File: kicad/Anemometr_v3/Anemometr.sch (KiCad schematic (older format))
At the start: 170 parts, among them J1 TxD, J10 +Z1, J11 +Z2, J12 +Z3, J13 +Z4, J14 -Z1, J15 -Z2, J16 -Z3, J17 -Z4, J18 1 TxD+, J19 2 TxD-, J2 RxD, J20 3 RxD+, J21 4-5, J22 6 RxD-, J23 7-8, J24 Conn_01x01_Female, J25 Conn_01x01_Female, J26 Conn_01x01_Female, J3 SCL, J4 SDA, J5 RST, J6 +EXT, J7 -EXT, J8 SWD, J9 SWC, Q1 5N10, U1 STM32F103C8Tx, U2 TS5A3166DBVR, U3 TS5A3166DBVR, U4 LMR14206, U5 TS5A3166DBVR, U6 NCP1117-3.3, U7 TS5A3166DBVR, U8 MCP1703-3.3, U9 MCP1703-3.3, Y1 CSTCE8M00G52A-R0, Y2 ECS-250-20-33

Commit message: изменено:      kicad/Anemometr_v3/Anemometr-cache.lib 	изменено:      kicad/Anemometr_v3/Anemometr-rescue.lib 	изменено:      kicad/Anemometr_v3/Anemometr.sch 	изменено:      kicad/Anemometr_v3/Anemometr.sch-bak 	изменено:      stm32cubeide/Anemometer/.settings/language.settings.xml
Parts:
- D20, D21: symbol My_Library:TLV3501-2 -> Anemometr-rescue:TLV3501-2-My_Library
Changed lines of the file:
@@
 Connection ~ 5900 3950
 $Comp
-L My_Library:TLV3501-2 D20
+L Anemometr-rescue:TLV3501-2-My_Library D20
 U 1 1 637C998F
 P 10050 1350
@@
 	10150 1600 10200 1600
 $Comp
-L My_Library:TLV3501-2 D21
+L Anemometr-rescue:TLV3501-2-My_Library D21
 U 1 1 638DF360
 P 10050 3150

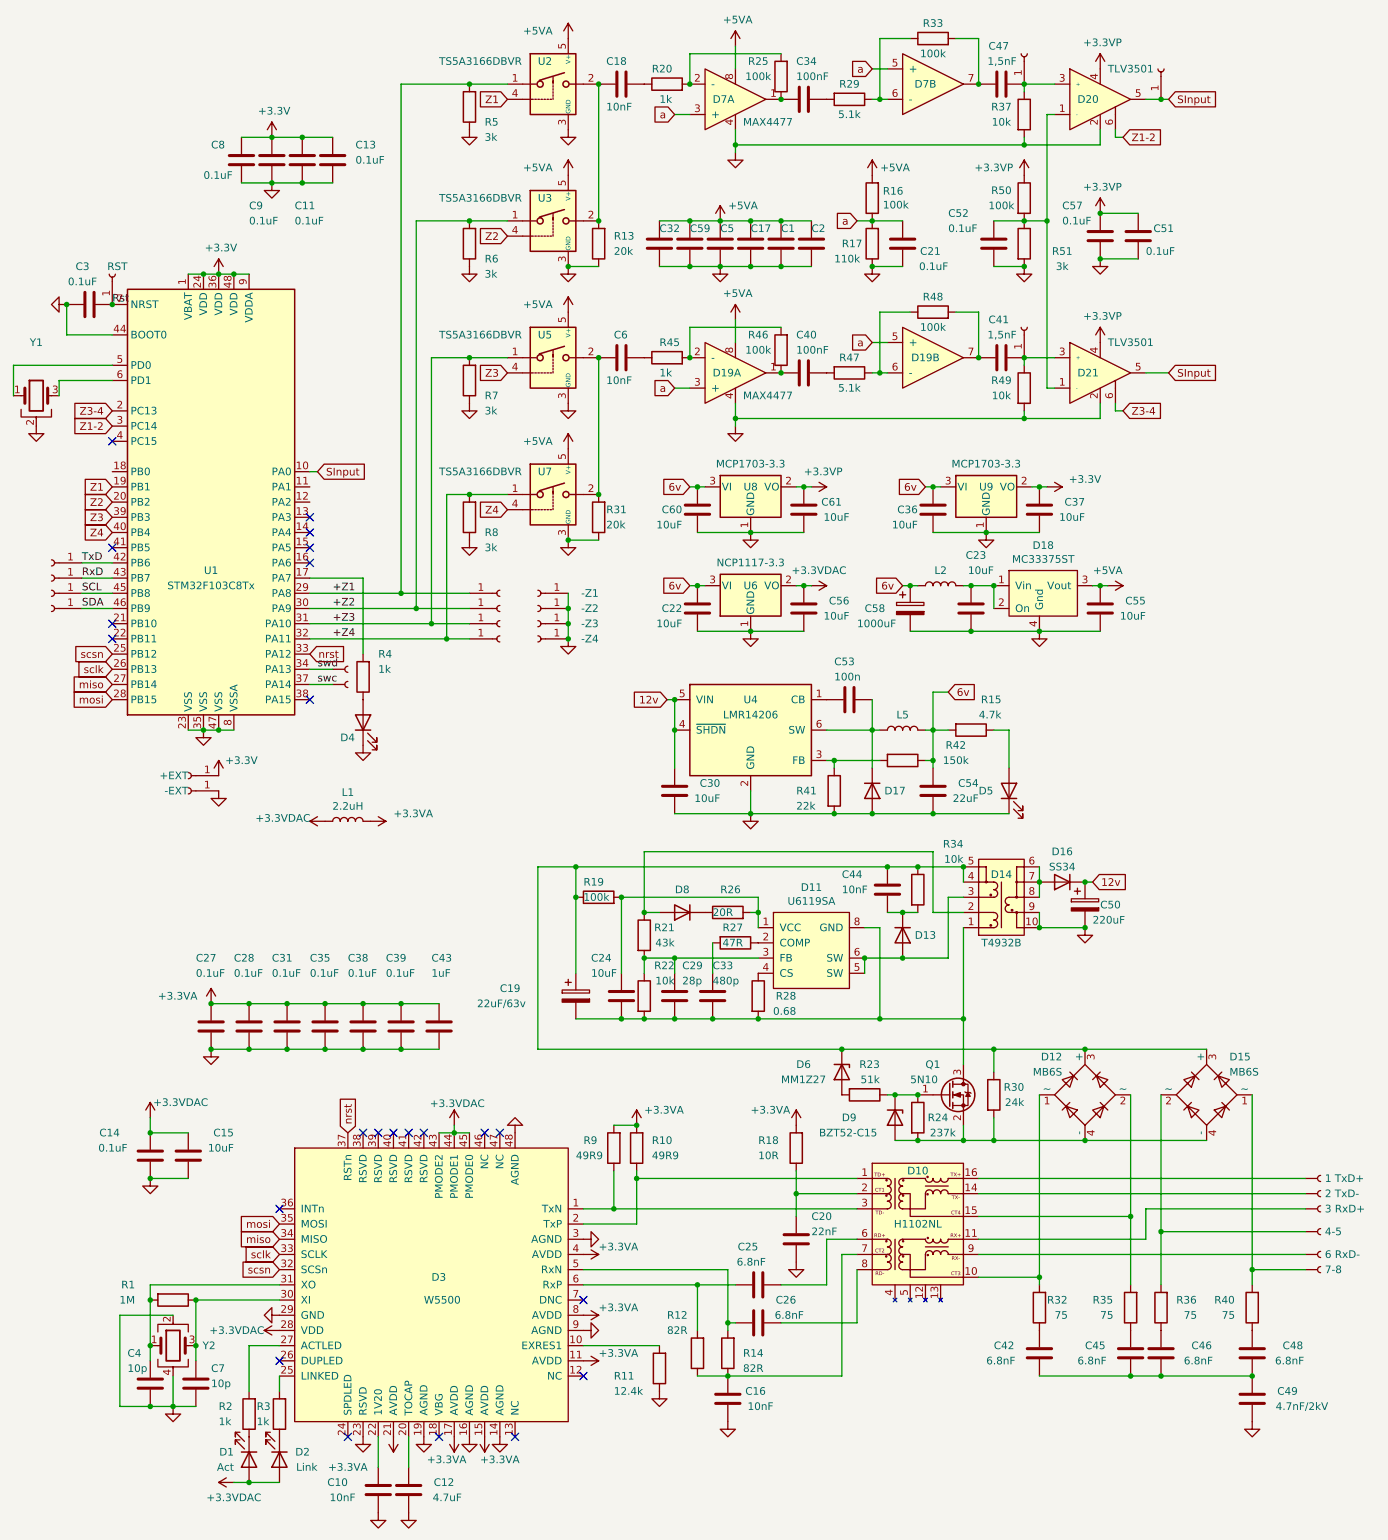
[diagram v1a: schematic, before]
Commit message: изменено:      kicad/Anemometr_v3/Anemometr-cache.lib 	изменено:      kicad/Anemometr_v3/Anemometr.kicad_pcb 	изменено:      kicad/Anemometr_v3/Anemometr.kicad_pcb-bak 	изменено:      kicad/Anemometr_v3/Anemometr.sch 	изменено:      kicad/Anemometr_v3/Anemometr.sch-bak
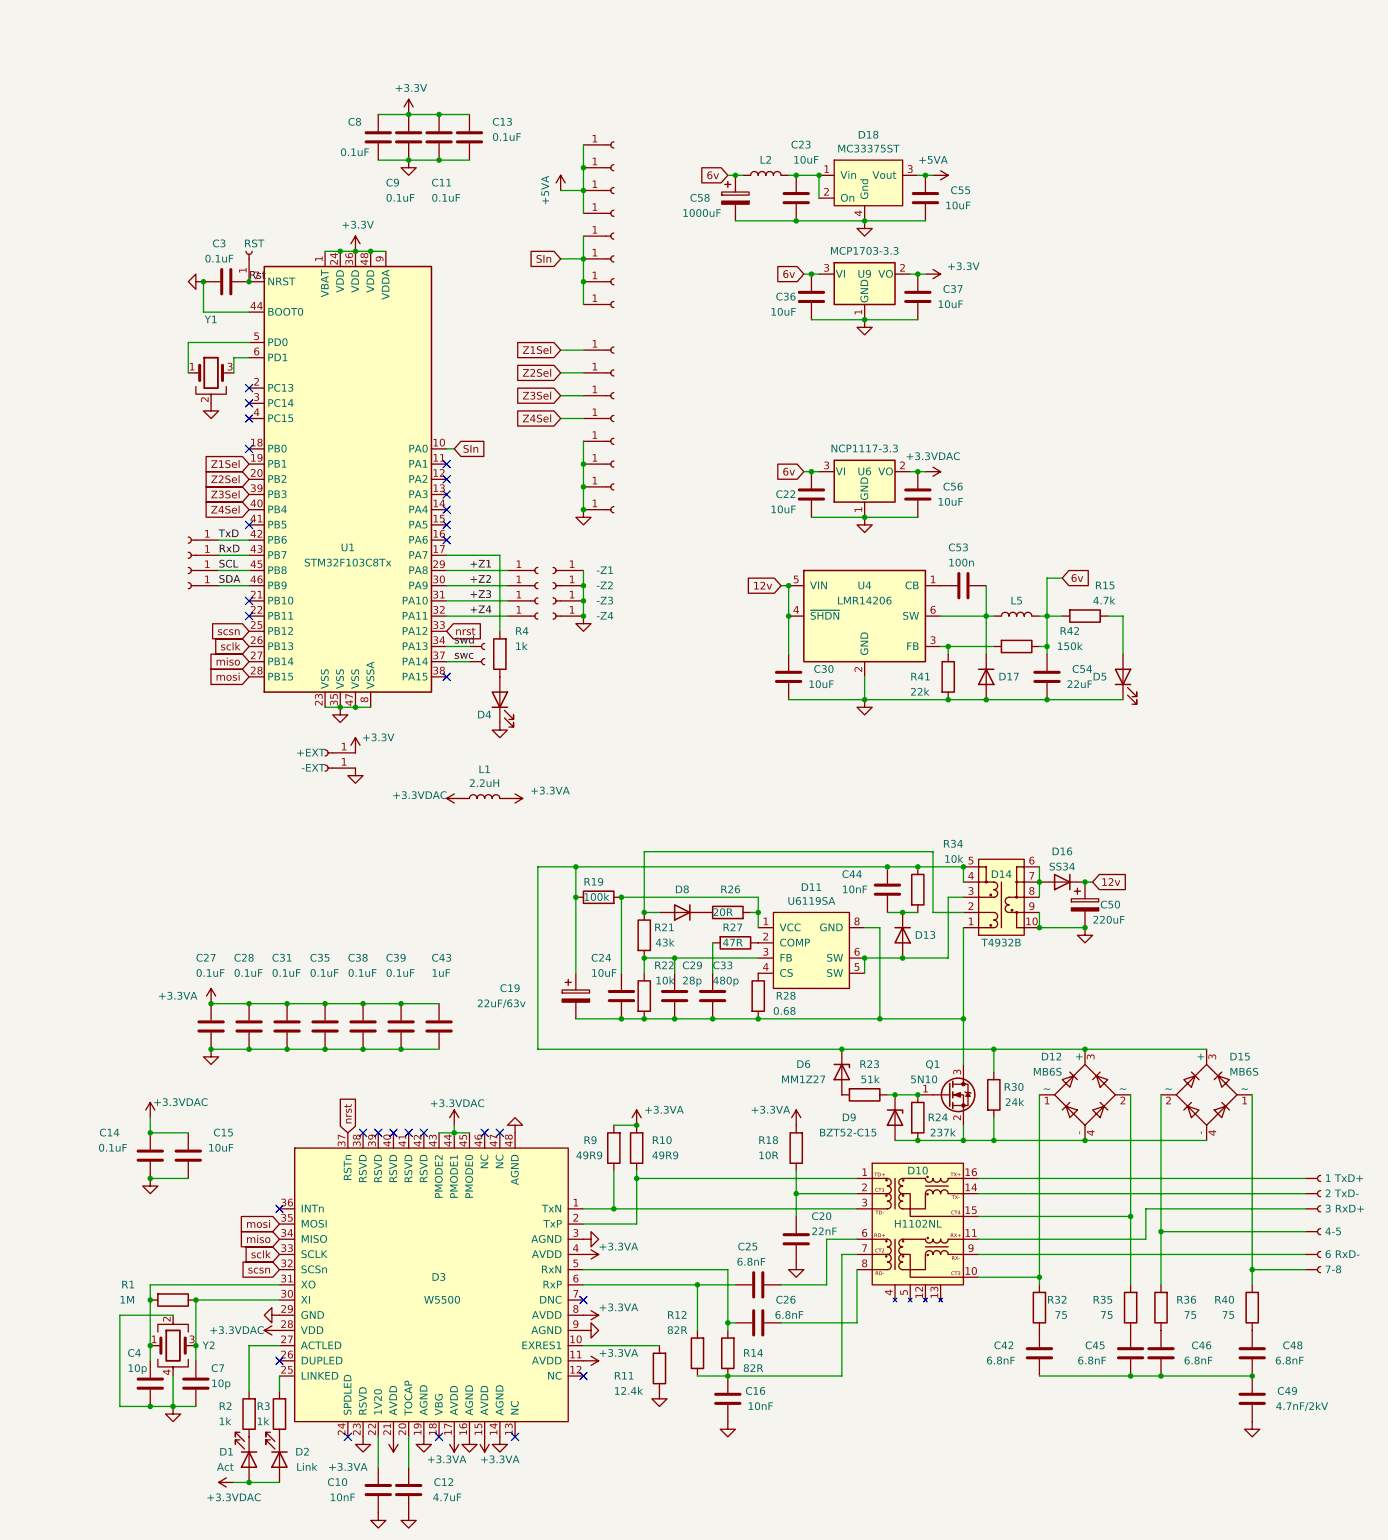
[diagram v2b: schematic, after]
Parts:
- removed C1, C17, C2, C21, C32, C5, C51, C52, C57, C59: 0.1uF, Capacitor_SMD:C_0402_1005Metric, symbol Device:C
- removed C18, C6: 10nF, Capacitor_SMD:C_0402_1005Metric, symbol Device:C
- removed C34, C40: 100nF, Capacitor_SMD:C_0402_1005Metric, symbol Device:C
- removed C41, C47: 1,5nF, Capacitor_SMD:C_0402_1005Metric, symbol Device:C
- removed C60, C61: 10uF, Capacitor_SMD:C_0805_2012Metric, symbol Device:C
- removed D19, D7: MAX4477, Package_SO:MSOP-8_3x3mm_P0.65mm, symbol Anemometr-rescue:MAX4477-My_Library
- removed D20, D21: TLV3501, Package_TO_SOT_SMD:SOT-23-6, symbol Anemometr-rescue:TLV3501-2-My_Library
- removed R13, R31: 20k, Resistor_SMD:R_0402_1005Metric, symbol Device:R
- removed R16, R25, R33, R46, R48, R50: 100k, Resistor_SMD:R_0402_1005Metric, symbol Device:R
- removed R17: 110k, Resistor_SMD:R_0402_1005Metric, symbol Device:R
- removed R20, R45: 1k, Resistor_SMD:R_0402_1005Metric, symbol Device:R
- removed R29, R47: 5.1k, Resistor_SMD:R_0402_1005Metric, symbol Device:R
- removed R37, R49: 10k, Resistor_SMD:R_0402_1005Metric, symbol Device:R
- removed R5, R51: 3k, Resistor_SMD:R_0402_1005Metric, symbol Device:R
- removed R6, R7, R8: 3k, Resistor_SMD:R_0603_1608Metric, symbol Device:R
- removed U2, U3, U5, U7: TS5A3166DBVR, Package_TO_SOT_SMD:SOT-23-5, symbol Analog_Switch:TS5A3166DBVR
- removed U8: MCP1703-3.3, Package_TO_SOT_SMD:SOT-23, symbol Regulator_Linear:MCP1700-3302E_SOT23
- added J27, J28, J29, J30, J31, J32, J33, J34, J35, J36, J37, J38, J39: +Z1, My-library:SMD-CONN, symbol Connector:Conn_01x01_Female
- J24, J25, J26: value Conn_01x01_Female -> +Z1; footprint My-library:ConnMini -> My-library:SMD-CONN
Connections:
- net +5VA: now also J24.1 (Pin_1), J25.1 (Pin_1), J26.1 (Pin_1), J27.1 (Pin_1)
- net GND: now also J36.1 (Pin_1), J37.1 (Pin_1), J38.1 (Pin_1), J39.1 (Pin_1)
- net SInput renamed SIn
- net SIn: now also J28.1 (Pin_1), J29.1 (Pin_1), J30.1 (Pin_1), J31.1 (Pin_1); no longer J24.1 (Pin_1)
- net Z1 renamed Z1Sel
- net Z1Sel: now also J32.1 (Pin_1)
- net Z1-2: no longer names the net of U1.3 (PC14)
- net Z2 renamed Z2Sel
- net Z2Sel: now also J33.1 (Pin_1)
- net Z3 renamed Z3Sel
- net Z3Sel: now also J34.1 (Pin_1)
- net Z3-4: no longer names the net of U1.2 (PC13)
- net Z4 renamed Z4Sel
- net Z4Sel: now also J35.1 (Pin_1)
- no-connect marks 23 -> 28
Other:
- moved on the sheet: C11, C13, C22, C23, C3, C30, C36, C37, C53, C54, C55, C56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

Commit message: изменено:      kicad/Anemometr_v3/Anemometr.sch 	изменено:      kicad/Anemometr_v3/Anemometr.sch-bak
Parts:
- D17: value SS56 -> SS56, VS10MQ060-M3/5
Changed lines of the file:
@@
 P 9300 5150
 F 0 "D17" V 9300 5300 50  0000 C CNN
-F 1 "SS56" V 9650 5150 50  0001 C CNN
+F 1 "SS56, VS10MQ060-M3/5" V 9650 5150 50  0001 C CNN
 F 2 "Diode_SMD:D_SMA" H 9300 5150 50  0001 C CNN
 F 3 "~" H 9300 5150 50  0001 C CNN
